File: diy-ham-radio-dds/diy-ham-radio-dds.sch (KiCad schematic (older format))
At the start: 63 parts, among them J1 ICSP, J2 I2C, J3 VCC, J4 NPN OUT, J5 , J6 UART_PROG, Q1 S0805, Q2 S0805, Q3 S0805, Q4 S0805, Q5 S0805, Q6 S0805, Q7 S0805, Q8 S0805, SW1 SW_Push, SW2 SW_Push, SW3 SW_Push, SW4 SW_Push, SW5 Rotary_Encoder_Switch, U1 ATmega328-AU, U2 74LS08, U3 L7805, U4 74HC595, Y1 16MHz

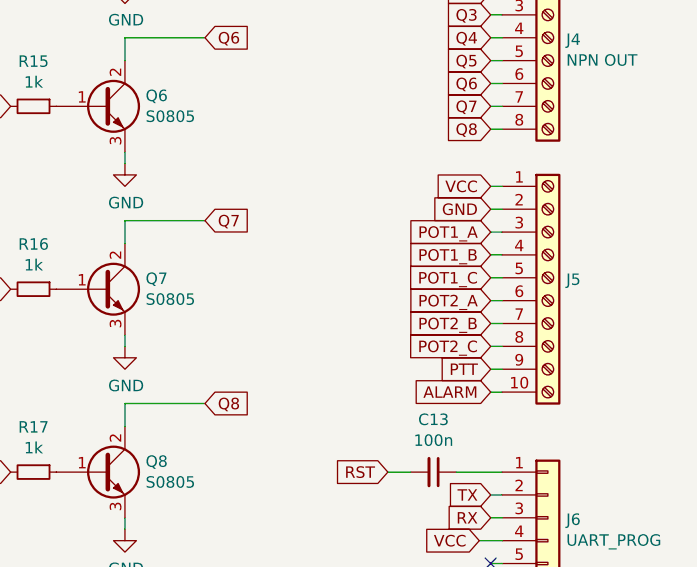
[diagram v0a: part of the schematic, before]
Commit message: Drawing in progress
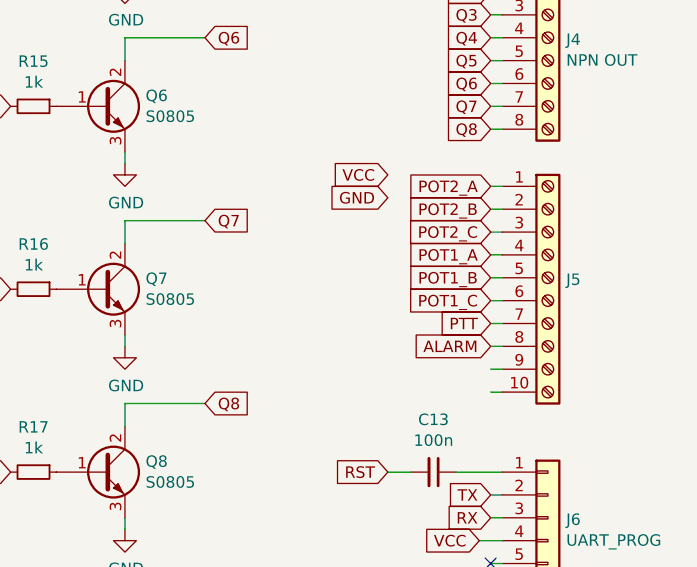
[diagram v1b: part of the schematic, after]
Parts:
- R2, R5: footprint Resistor_SMD:R_0402_1005Metric_Pad0.72x0.64mm_HandSolder -> Resistor_SMD:R_0402_1005Metric
- R3: footprint Resistor_SMD:R_01005_0402Metric -> Resistor_SMD:R_0402_1005Metric
- R6: footprint Resistor_SMD:R_01005_0402Metric_Pad0.57x0.30mm_HandSolder -> Resistor_SMD:R_0402_1005Metric
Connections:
- net ALARM: now also J5.8 (Pin_8); no longer J5.10 (Pin_10)
- net GND: no longer J5.2 (Pin_2)
- net POT1_A: now also J5.4 (Pin_4); no longer J5.3 (Pin_3)
- net POT1_B: now also J5.5 (Pin_5); no longer J5.4 (Pin_4)
- net POT1_C: now also J5.6 (Pin_6); no longer J5.5 (Pin_5)
- net POT2_A: now also J5.1 (Pin_1); no longer J5.6 (Pin_6)
- net POT2_B: now also J5.2 (Pin_2); no longer J5.7 (Pin_7)
- net POT2_C: now also J5.3 (Pin_3); no longer J5.8 (Pin_8)
- net PTT: now also J5.7 (Pin_7); no longer J5.9 (Pin_9)
- net VCC: no longer J5.1 (Pin_1)
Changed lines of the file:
@@
 F 0 "R6" H 5559 4496 50  0000 L CNN
 F 1 "220R 1/8W" H 5559 4405 50  0000 L CNN
-F 2 "Resistor_SMD:R_01005_0402Metric_Pad0.57x0.30mm_HandSolder" H 5500 4450 50  0001 C CNN
+F 2 "Resistor_SMD:R_0402_1005Metric" H 5500 4450 50  0001 C CNN
 F 3 "~" H 5500 4450 50  0001 C CNN
 	1    5500 4450
@@
 F 0 "R2" V 3246 2750 50  0000 C CNN
 F 1 "1k" V 3155 2750 50  0000 C CNN
-F 2 "Resistor_SMD:R_0402_1005Metric_Pad0.72x0.64mm_HandSolder" H 3050 2750 50  0001 C CNN
+F 2 "Resistor_SMD:R_0402_1005Metric" H 3050 2750 50  0001 C CNN
 F 3 "~" H 3050 2750 50  0001 C CNN
 	1    3050 2750
@@
 F 0 "R3" V 2946 2950 50  0000 C CNN
 F 1 "1k" V 2855 2950 50  0000 C CNN
-F 2 "Resistor_SMD:R_01005_0402Metric" H 3050 2950 50  0001 C CNN
+F 2 "Resistor_SMD:R_0402_1005Metric" H 3050 2950 50  0001 C CNN
 F 3 "~" H 3050 2950 50  0001 C CNN
 	1    3050 2950
@@
 NoConn ~ 3000 7450
 NoConn ~ 3000 7650
+Text GLabel 9500 3900 0    50   Input ~ 0
+VCC
+Text GLabel 9500 4000 0    50   Input ~ 0
+GND
+Text GLabel 9950 4250 0    50   Input ~ 0
+POT1_A
+Text GLabel 9950 4350 0    50   Input ~ 0
+POT1_B
+Text GLabel 9950 4450 0    50   Input ~ 0
+POT1_C
 Text GLabel 9950 3950 0    50   Input ~ 0
-VCC
+POT2_A
 Text GLabel 9950 4050 0    50   Input ~ 0
-GND
+POT2_B
 Text GLabel 9950 4150 0    50   Input ~ 0
-POT1_A
-Text GLabel 9950 4250 0    50   Input ~ 0
-POT1_B
-Text GLabel 9950 4350 0    50   Input ~ 0
-POT1_C
-Text GLabel 9950 4450 0    50   Input ~ 0
-POT2_A
-Text GLabel 9950 4550 0    50   Input ~ 0
-POT2_B
-Text GLabel 9950 4650 0    50   Input ~ 0
 POT2_C
 $Comp
@@
 F 0 "R5" V 4296 3700 50  0000 C CNN
 F 1 "100R" V 4205 3700 50  0000 C CNN
-F 2 "Resistor_SMD:R_0402_1005Metric_Pad0.72x0.64mm_HandSolder" H 4400 3700 50  0001 C CNN
+F 2 "Resistor_SMD:R_0402_1005Metric" H 4400 3700 50  0001 C CNN
 F 3 "~" H 4400 3700 50  0001 C CNN
 	1    4400 3700
@@
 Text GLabel 4500 3700 2    50   Input ~ 0
 ALARM
-Text GLabel 9950 4750 0    50   Input ~ 0
+Text GLabel 9950 4550 0    50   Input ~ 0
 PTT
-Text GLabel 9950 4850 0    50   Input ~ 0
+Text GLabel 9950 4650 0    50   Input ~ 0
 ALARM
 Text GLabel 5800 6350 2    50   Input ~ 0
